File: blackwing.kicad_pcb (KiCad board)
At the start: 2 copper layers, 161.9 x 119.1 mm, 36 parts, among them J1 Conn_01x04, SW00 SW_Push, SW01 SW_Push, SW02 SW_Push, SW03 SW_Push, SW04 SW_Push, SW05 SW_Push, SW10 SW_Push, SW11 SW_Push, SW12 SW_Push, SW13 SW_Push, SW14 SW_Push, SW15 SW_Push, SW20 SW_Push, SW21 SW_Push, SW22 SW_Push, SW23 SW_Push, SW24 SW_Push, SW25 SW_Push, SW30 SW_Push, SW31 SW_Push, SW32 SW_Push, SW33 SW_Push, SW34 SW_Push, SW35 SW_Push, SW40 SW_Push, SW41 SW_Push, SW42 SW_Push, SW43 SW_Push, SW44 SW_Push, SW45 SW_Push, SW50 SW_Push, U1 CORE51822, U2 CORE51822

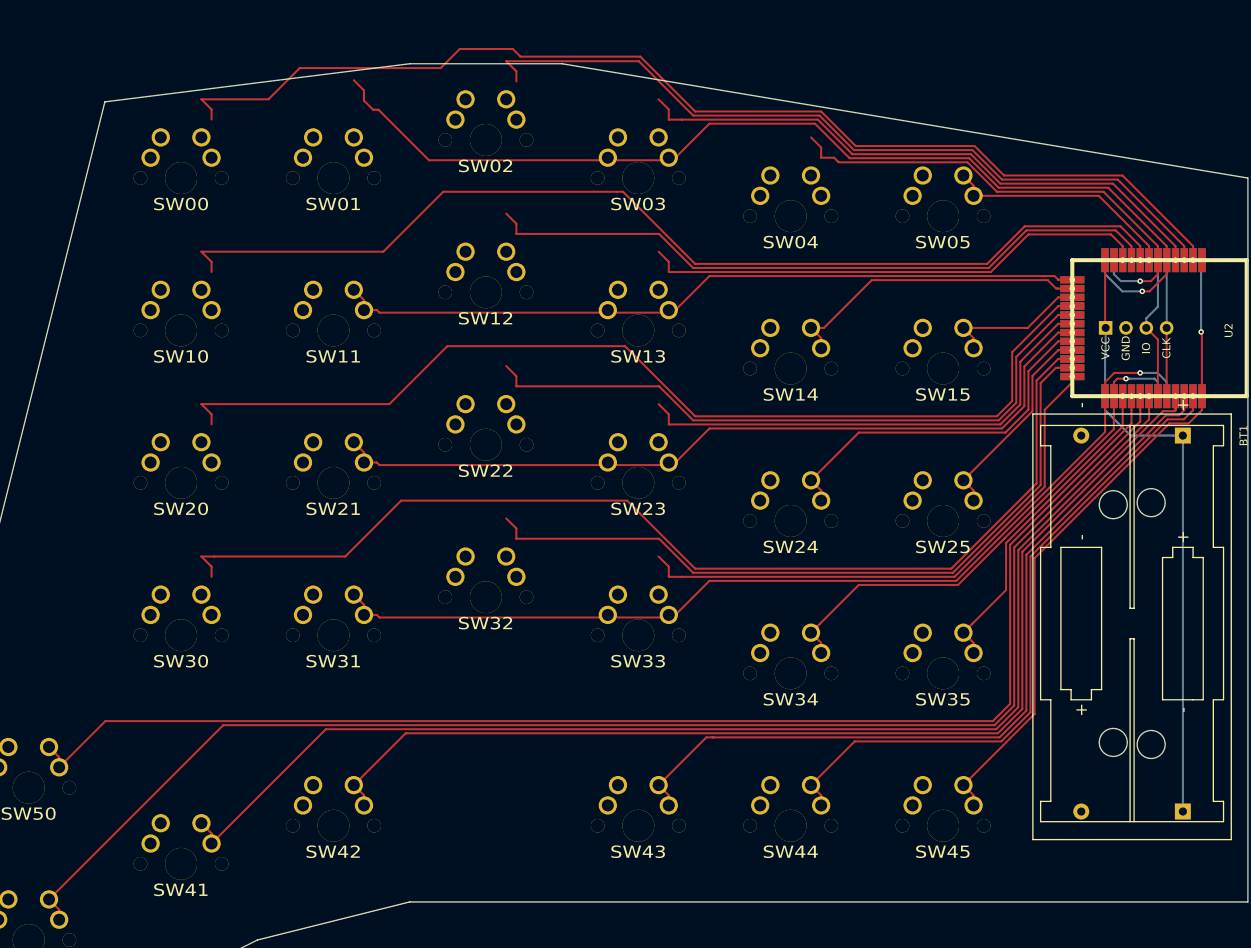
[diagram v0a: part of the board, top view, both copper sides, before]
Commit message: try
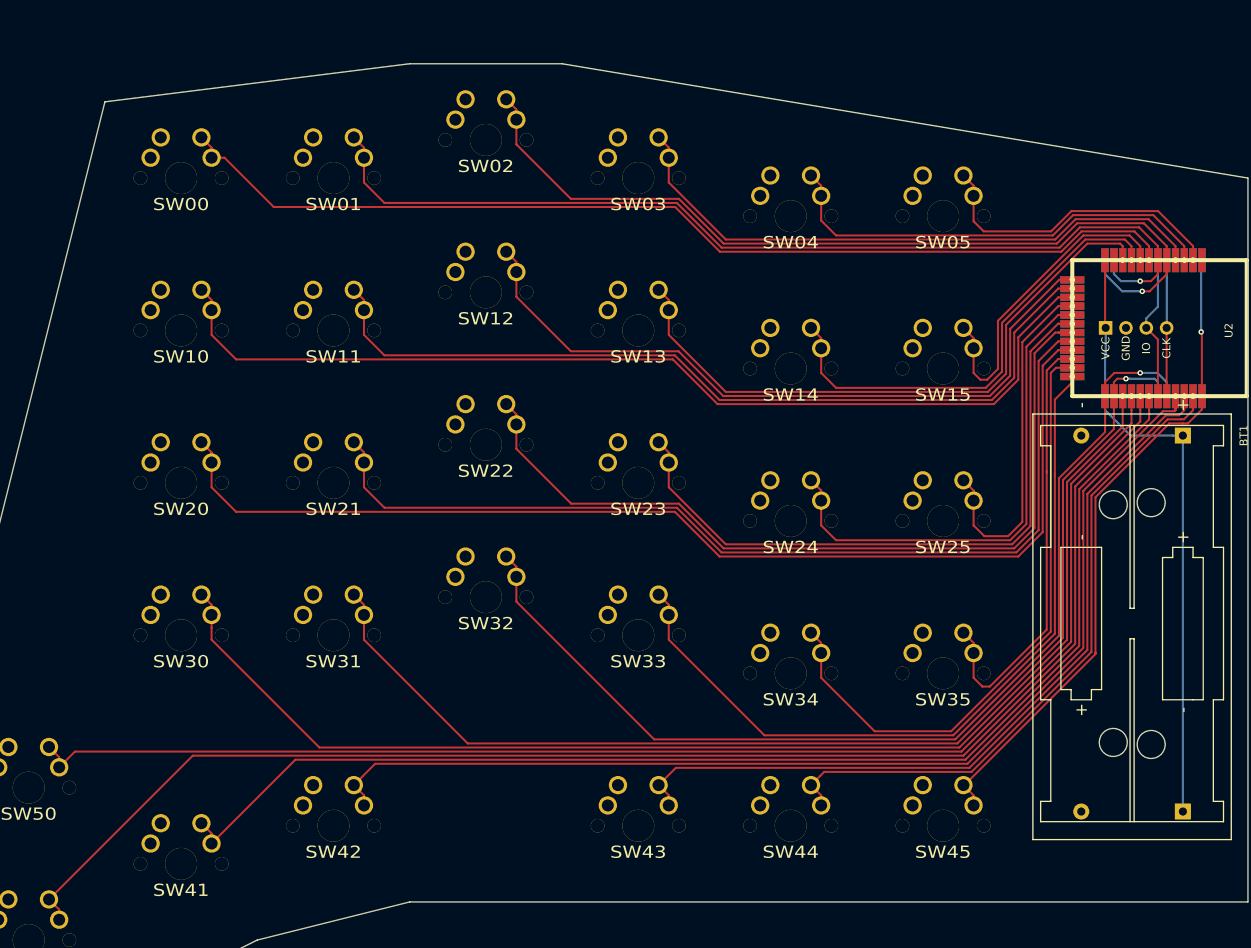
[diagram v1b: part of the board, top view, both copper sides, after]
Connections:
- U1 pad 10: S35 -> S30
- U1 pad 14: S32 -> S34
- U1 pad 15: S30 -> S35
- U1 pad 16: S25 -> S20
- U1 pad 17: S24 -> S21
- U1 pad 18: S21 -> S22
- U1 pad 20: S22 -> S24
- U1 pad 21: S20 -> S25
- U1 pad 22: S15 -> S10
- U1 pad 23: S14 -> S11
- U1 pad 24: S11 -> S12
- U1 pad 25: S01 -> S02
- U1 pad 26: S04 -> S01
- U1 pad 28: S12 -> S14
- U1 pad 29: S10 -> S15
- U1 pad 30: S05 -> S00
- U1 pad 34: S02 -> S04
- U1 pad 35: S00 -> S05
- U1 pad 5: S31 -> S32
- U1 pad 6: S34 -> S31
- U2 pad 13: S11 -> S12
- U2 pad 14: S14 -> S11
- U2 pad 15: S15 -> S10
- U2 pad 16: S20 -> S25
- U2 pad 17: S22 -> S24
- U2 pad 19: S21 -> S22
- U2 pad 2: S00 -> S05
- U2 pad 20: S24 -> S21
- U2 pad 21: S25 -> S20
- U2 pad 22: S30 -> S35
- U2 pad 23: S32 -> S34
- U2 pad 25: S31 -> S32
- U2 pad 26: S34 -> S31
- U2 pad 27: S35 -> S30
- U2 pad 3: S02 -> S04
- U2 pad 5: S01 -> S02
- U2 pad 6: S04 -> S01
- U2 pad 7: S05 -> S00
- U2 pad 8: S10 -> S15
- U2 pad 9: S12 -> S14
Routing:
- net S32: track 92.4 -> 131.0 mm
- net S33: track 69.9 -> 98.1 mm
- net S31: track 122.1 -> 146.6 mm
- net S23: track 61.8 -> 85.5 mm
- net S22: track 83.1 -> 106.5 mm
- net S15: track 18.3 -> 40.6 mm
- net S30: track 136.7 -> 157.6 mm
- net S14: track 38.6 -> 59.1 mm
- net S21: track 101.5 -> 121.4 mm
- net S25: track 26.0 -> 44.1 mm
- net S24: track 45.7 -> 63.0 mm
- net S13: track 64.1 -> 79.0 mm
- net S35: track 40.9 -> 55.1 mm
- net S11: track 93.8 -> 107.1 mm
- net S34: track 64.9 -> 78.1 mm
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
